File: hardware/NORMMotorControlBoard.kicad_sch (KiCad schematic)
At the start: 32 parts, among them J1 Front Right Motor, J2 Front Left Motor, J3 Back Right Motor, J4 Back Left Motor, J5 Conn_01x02_Socket, J6 SparePins, J7 SparePins, SW1 Reset, U1 Front Driver, U2 Back Driver, U3 74HC595

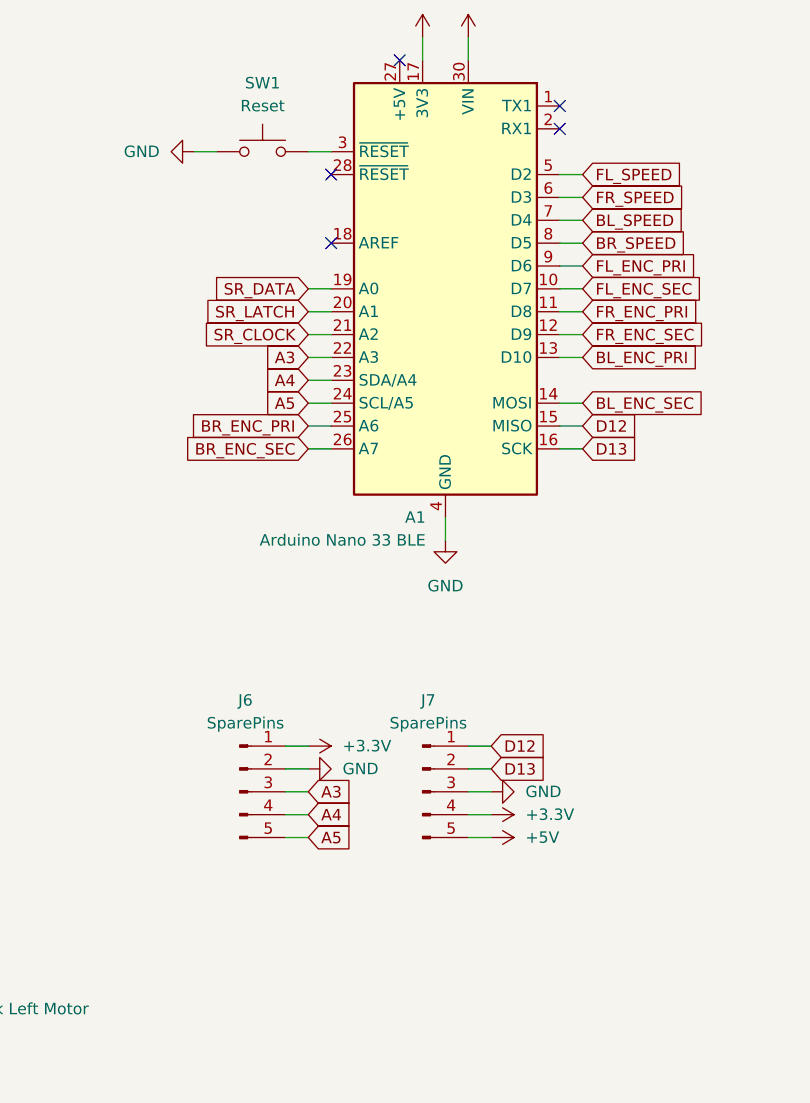
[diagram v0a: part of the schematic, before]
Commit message: V1.3
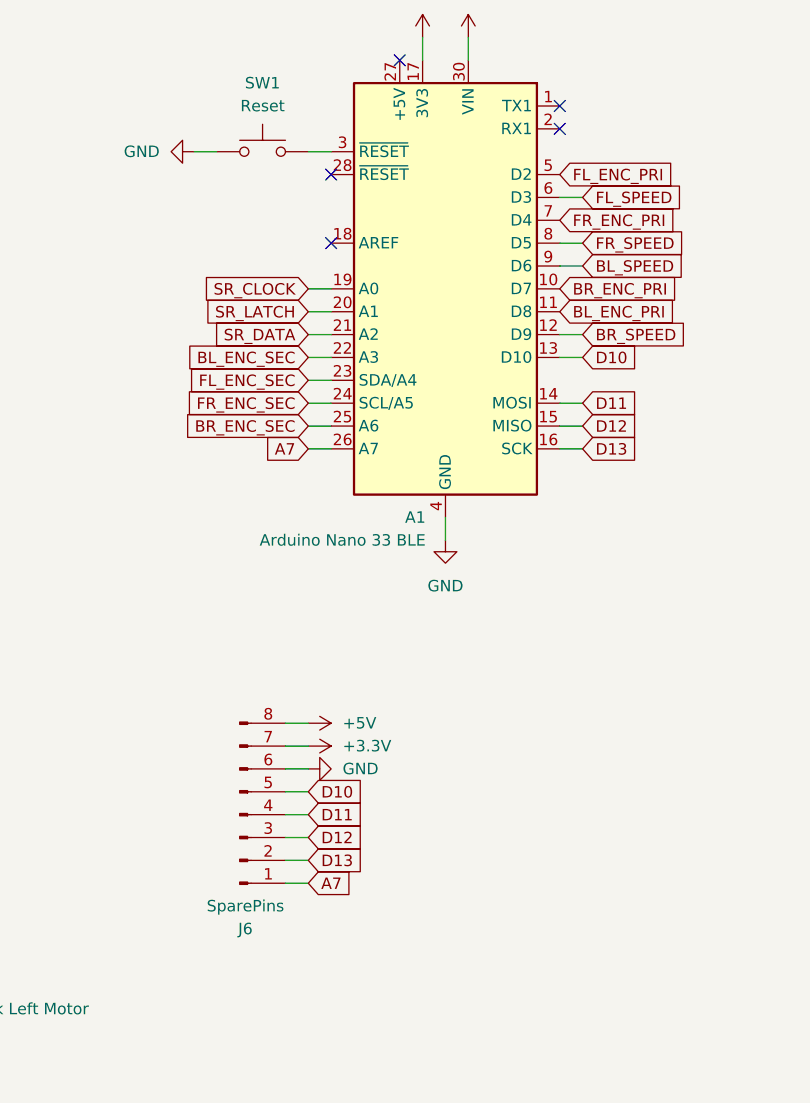
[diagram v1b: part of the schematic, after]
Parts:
- removed J7: SparePins, Connector_PinHeader_2.54mm:PinHeader_1x05_P2.54mm_Vertical, symbol Connector:Conn_01x05_Pin
- J6: footprint Connector_PinHeader_2.54mm:PinHeader_1x05_P2.54mm_Horizontal -> Connector_PinHeader_2.54mm:PinHeader_1x08_P2.54mm_Horizontal; symbol Connector:Conn_01x05_Pin -> Connector:Conn_01x08_Pin
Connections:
- net +3.3V: now also J6.7 (Pin_7); no longer J6.1 (Pin_1)
- net +5V: now also J6.8 (Pin_8)
- net BL_ENC_PRI: now also A1.11 (D8); no longer A1.13 (D10)
- net BL_ENC_SEC: now also A1.22 (A3); no longer A1.14 (MOSI)
- net BL_SPEED: now also A1.9 (D6); no longer A1.7 (D4)
- net BR_ENC_PRI: now also A1.10 (D7); no longer A1.25 (A6)
- net BR_ENC_SEC: now also A1.25 (A6); no longer A1.26 (A7)
- net BR_SPEED: now also A1.12 (D9); no longer A1.8 (D5)
- net D12: now also J6.3 (Pin_3)
- net D13: now also J6.2 (Pin_2)
- net FL_ENC_PRI: now also A1.5 (D2); no longer A1.9 (D6)
- net FL_ENC_SEC: now also A1.23 (SDA/A4); no longer A1.10 (D7)
- net FL_SPEED: now also A1.6 (D3); no longer A1.5 (D2)
- net FR_ENC_PRI: now also A1.7 (D4); no longer A1.11 (D8)
- net FR_ENC_SEC: now also A1.24 (SCL/A5); no longer A1.12 (D9)
- net FR_SPEED: now also A1.8 (D5); no longer A1.6 (D3)
- net GND: now also J6.6 (Pin_6); no longer J6.2 (Pin_2)
- net SR_CLOCK: now also A1.19 (A0); no longer A1.21 (A2)
- net SR_DATA: now also A1.21 (A2); no longer A1.19 (A0)
- removed net A3: A1.22 (A3), J6.3 (Pin_3)
- net A4 renamed D11
- net D11: now also A1.14 (MOSI); no longer A1.23 (SDA/A4)
- net A5 renamed D10
- net D10: now also A1.13 (D10); no longer A1.24 (SCL/A5)
- new net A7: A1.26 (A7), J6.1 (Pin_1)
